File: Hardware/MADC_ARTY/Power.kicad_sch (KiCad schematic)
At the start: 11 parts, among them U27 TSR2-2450, U5 ADP5070AREZ, U7 ADP7142ARDZ-3.3

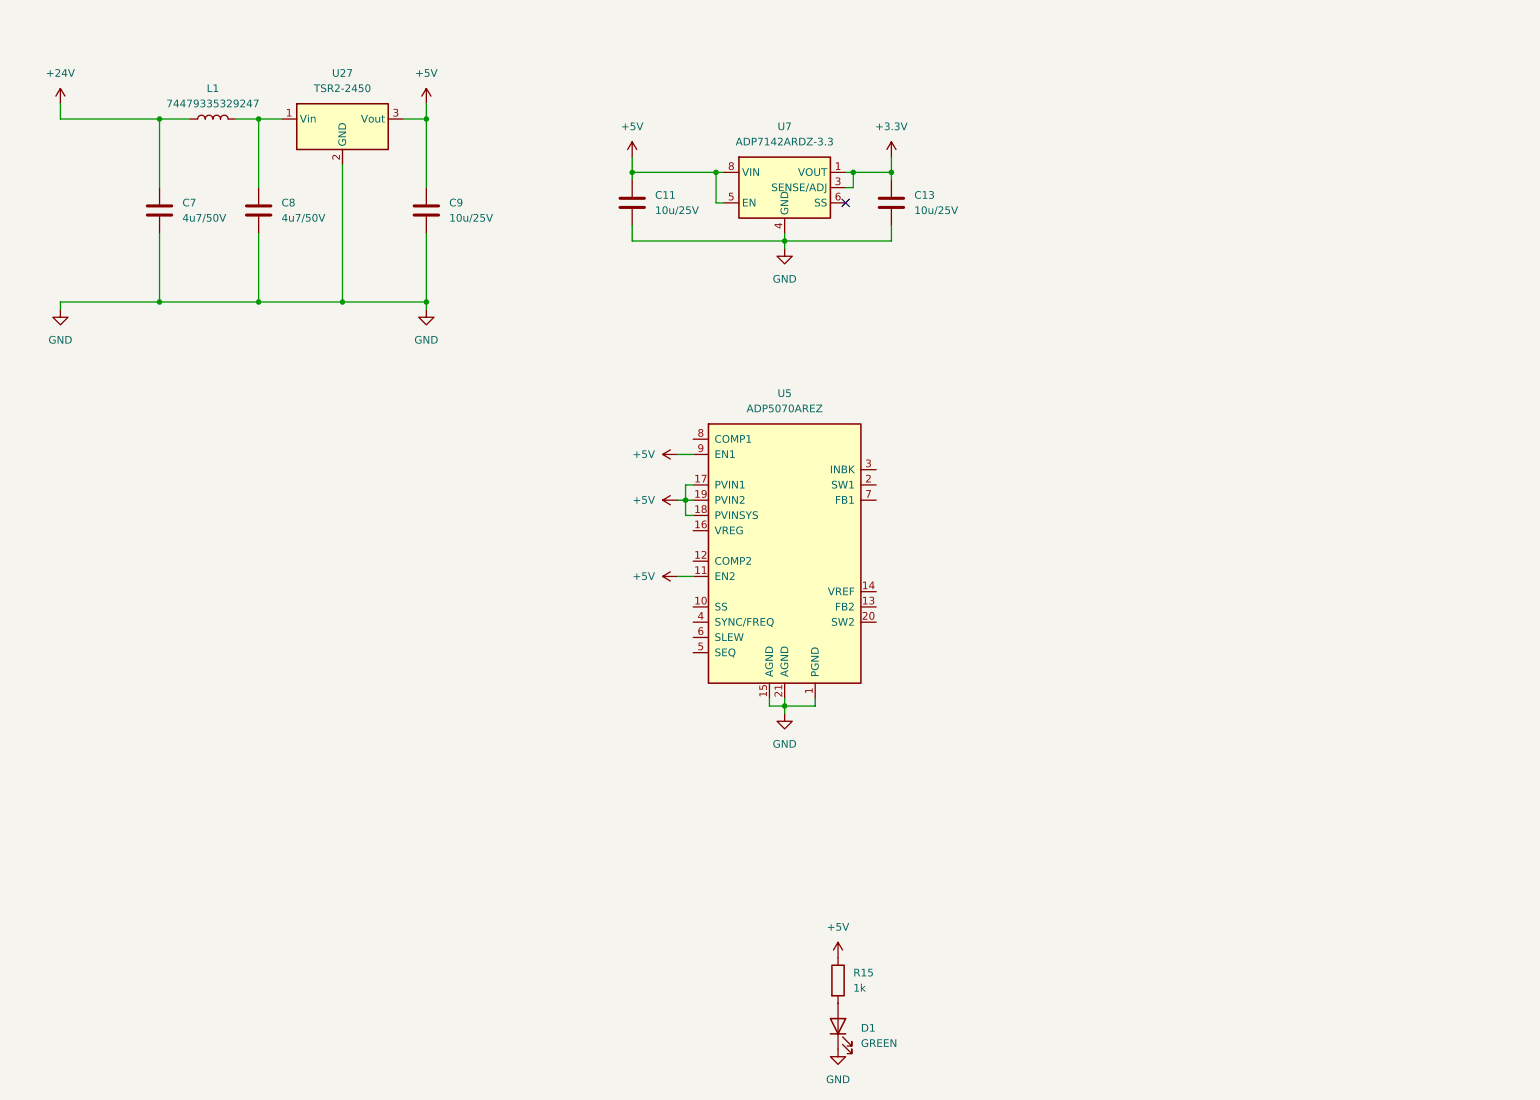
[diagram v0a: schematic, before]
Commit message: Schematic
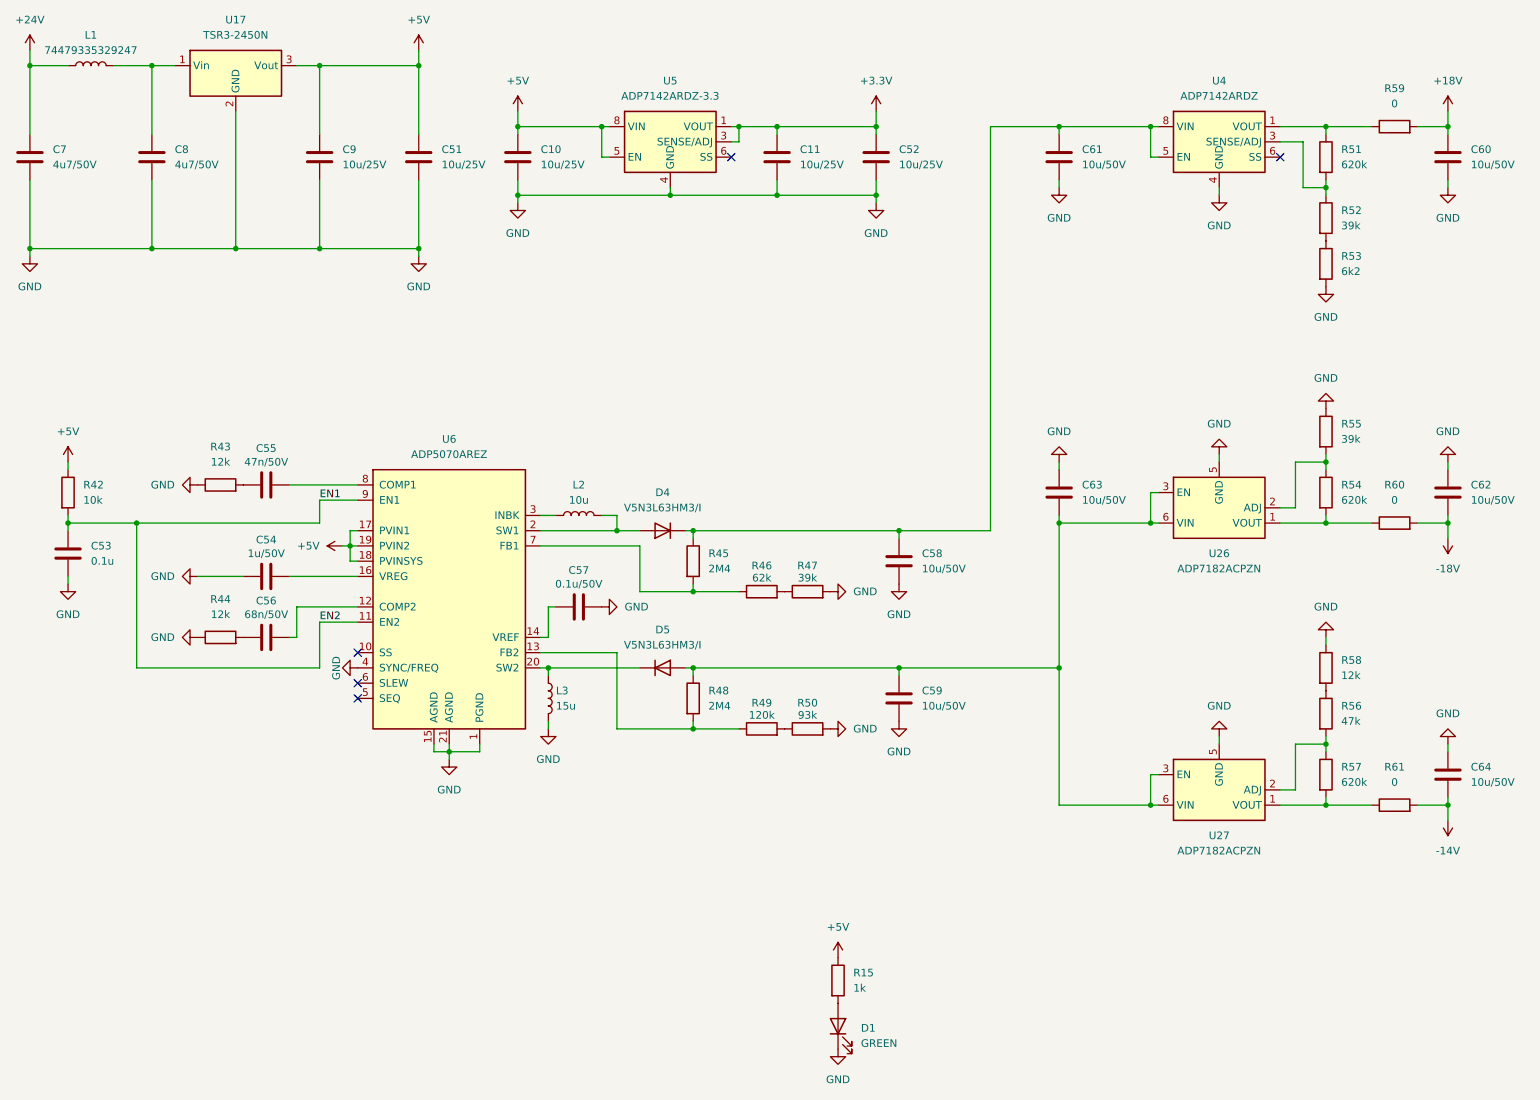
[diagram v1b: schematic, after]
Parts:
- removed U27: TSR2-2450, Converter_DCDC:Converter_DCDC_TRACO_TSR2-xxxx_THT, symbol Regulator_Switching:TSR2-2450
- added C51, C52: 10u/25V, Capacitor_SMD:C_1206_3216Metric, symbol Device:C
- added C53: 0.1u, symbol Device:C
- added C54: 1u/50V, symbol Device:C
- added C55: 47n/50V, symbol Device:C
- added C56: 68n/50V, symbol Device:C
- added C57: 0.1u/50V, symbol Device:C
- added C58, C59, C60, C61, C62, C63, C64: 10u/50V, Capacitor_SMD:C_1206_3216Metric, symbol Device:C
- added D4, D5: V5N3L63HM3/I, symbol Device:D
- added L2: 10u, symbol Device:L
- added L3: 15u, symbol Device:L
- added R42: 10k, symbol Device:R
- added R43, R44, R58: 12k, symbol Device:R
- added R45, R48: 2M4, symbol Device:R
- added R46: 62k, symbol Device:R
- added R47, R52, R55: 39k, symbol Device:R
- added R49: 120k, symbol Device:R
- added R50: 93k, symbol Device:R
- added R51, R54, R57: 620k, symbol Device:R
- added R53: 6k2, symbol Device:R
- added R56: 47k, symbol Device:R
- added R59, R60, R61: 0, symbol Device:R
- added U17: TSR3-2450N, Converter_DCDC:Converter_DCDC_TRACO_TSR2-24xxN_TSR2-24xxxN_THT, symbol Regulator_Switching:TSR3-2450N
- added U26, U27: ADP7182ACPZN, Package_CSP:LFCSP-6-1EP_2x2mm_P0.65mm_EP1x1.6mm, symbol MADC_ARTY:ADP7182ACPZN
- added U4: ADP7142ARDZ, Package_SO:SOIC-8-1EP_3.9x4.9mm_P1.27mm_EP2.29x3mm, symbol Regulator_Linear:ADP7142ARDZ
- renumbered C11 to C10, C13 to C11, U7 to U5, U5 to U6
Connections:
- net +3.3V: now also C52.1
- net +5V: now also C51.1, R42.1, U17.3 (Vout); no longer U6.11 (EN2), U6.9 (EN1)
- net GND: now also U6.4 (SYNC/FREQ), C51.2, C52.2, C53.2, C54.1, C57.2, C58.2, C59.2, C60.2, C61.2, C62.1, C63.1, C64.1, L3.2, R43.1, R44.1, R47.2, R50.2, R53.2, R55.1, R58.1, U17.2 (GND), U26.5 (GND), U27.5 (GND), U4.4 (GND), U4.9 (GND)
- net at U6.12 (COMP2): now also C56.2
- net at U6.13 (FB2): now also R48.2, R49.1
- net at U6.14 (VREF): now also C57.1
- net at U6.16 (VREG): now also C54.2
- net at U6.2 (SW1): now also D4.2 (A), L2.2
- net at U6.20 (SW2): now also D5.1 (K), L3.1
- net at U6.3 (INBK): now also L2.1
- net at U6.7 (FB1): now also R45.2, R46.1
- net at U6.8 (COMP1): now also C55.2
- net at C8.1, L1.2: now also U17.1 (Vin)
- new net: R49.2, R50.1
- new net: R54.1, R55.2, U26.2 (ADJ)
- new net: R54.2, R60.1, U26.1 (VOUT)
- new net: R57.2, R61.1, U27.1 (VOUT)
- new net: R56.2, R57.1, U27.2 (ADJ)
- new net: R51.1, R59.1, U4.1 (VOUT), U4.2 (VOUT)
- new net: C58.1, C61.1, D4.1 (K), R45.1, U4.5 (EN), U4.7 (VIN), U4.8 (VIN)
- new net: R46.2, R47.1
- new net: C56.1, R44.2
- new net: C55.1, R43.2
- new net: R51.2, R52.1, U4.3 (SENSE/ADJ)
- new net: R56.1, R58.2
- new net: R52.2, R53.1
- new net +18V: C60.1, R59.2
- new net -14V: C64.2, R61.2
- new net -18V: C62.2, R60.2
- new net EN1: C53.1, R42.2, U6.11 (EN2), U6.9 (EN1)
- new net EPAD: C59.1, C63.2, D5.2 (A), R48.1, U26.3 (EN), U26.6 (VIN), U26.7 (EPAD), U27.3 (EN), U27.6 (VIN), U27.7 (EPAD)
- no-connect marks 1 -> 5
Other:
- moved on the sheet: C10, C11, C7, C8, C9, L1, U5, U6
